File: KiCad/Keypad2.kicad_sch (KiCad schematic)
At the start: 22 parts, among them J1 Keypad, J2 USB-C, U1 ESP32-PICO-MINI-02, U2 SP3485, U3 FT231XQ, U4 LMR16006+FB

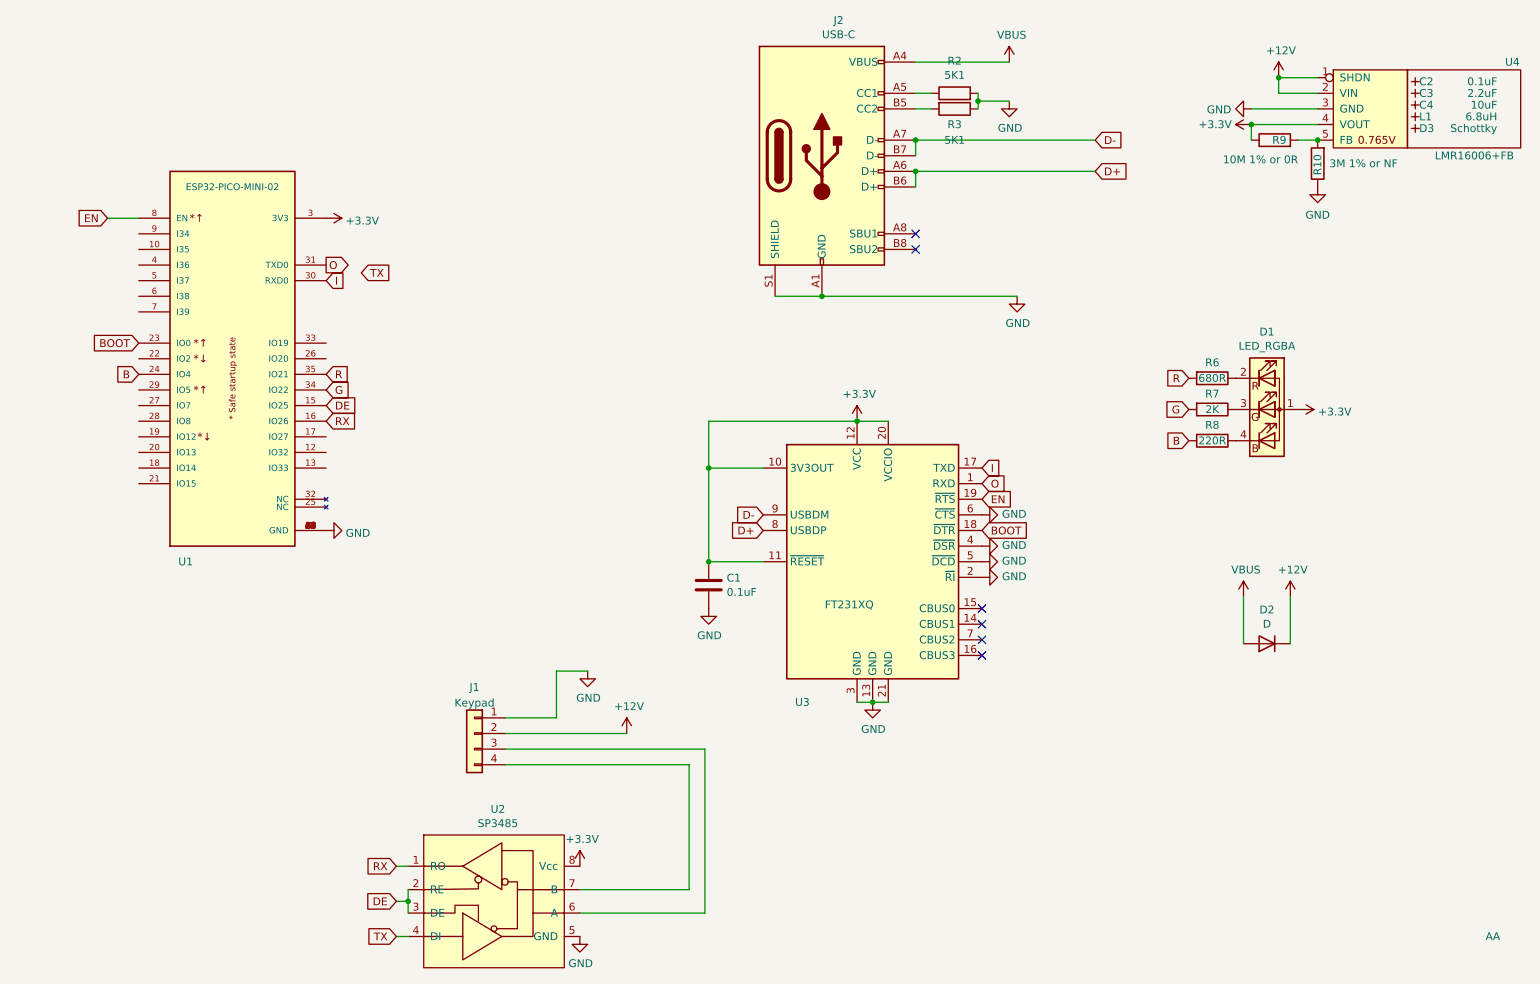
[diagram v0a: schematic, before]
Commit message: Keypad2
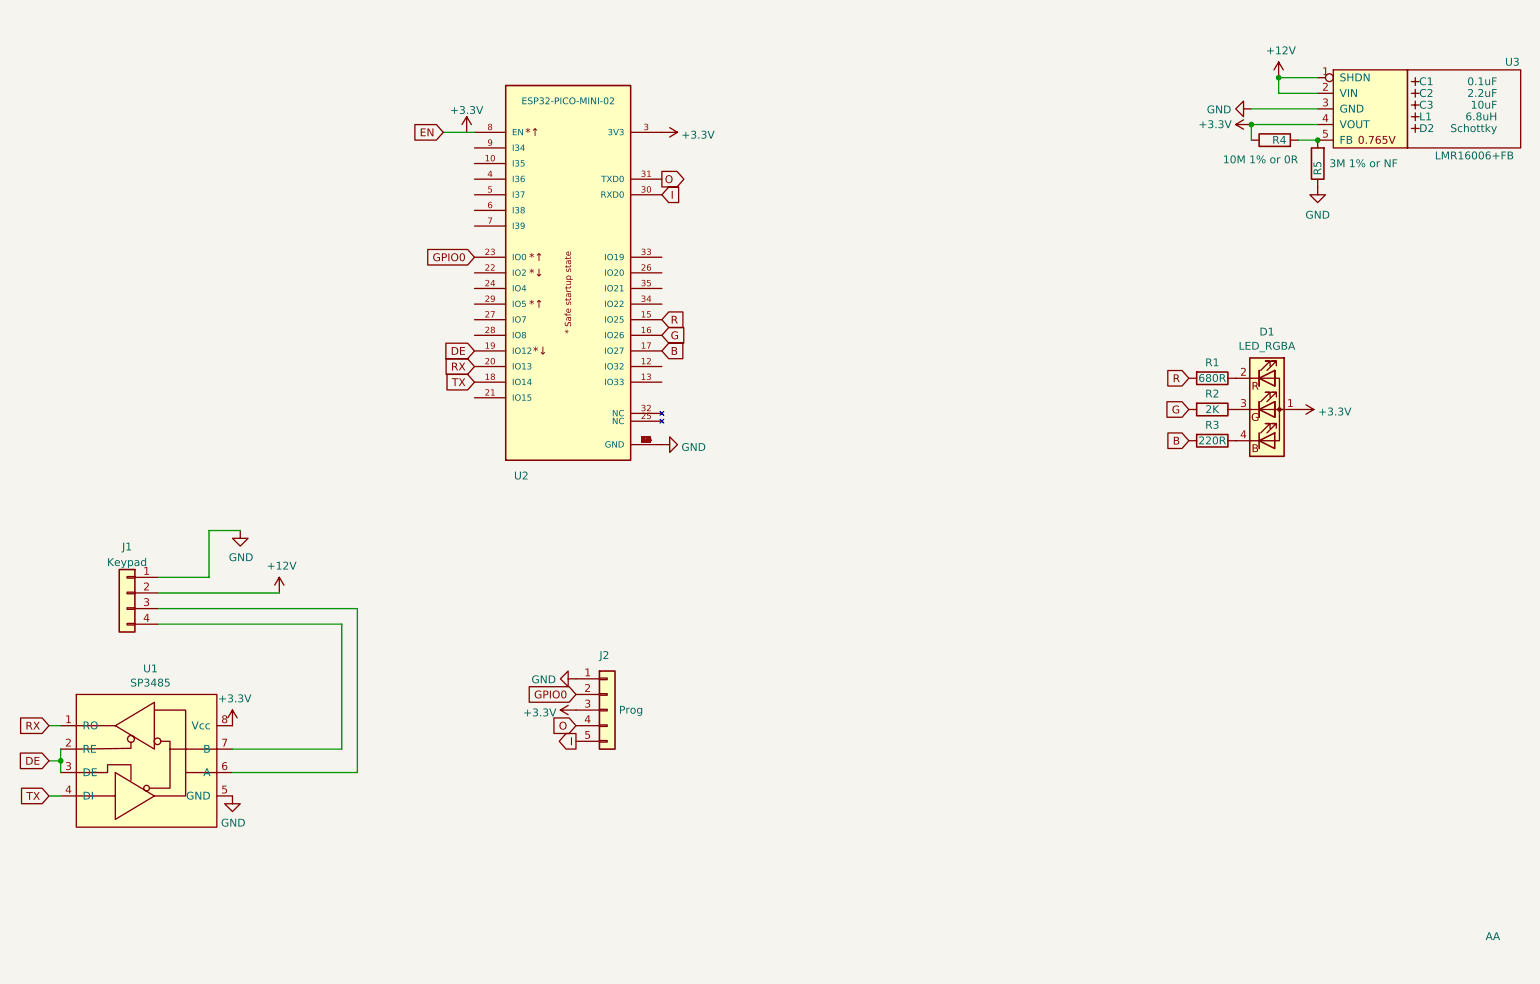
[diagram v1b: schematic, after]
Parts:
- removed C1: 0.1uF, RevK:C_0603, symbol Device:C
- removed D2: D, Diode_SMD:D_1206_3216Metric_Pad1.42x1.75mm_HandSolder, symbol Device:D
- removed J2: USB-C, RevK:USC16-TR-Round, symbol Connector:USB_C_Receptacle_USB2.0
- removed R2, R3: 5K1, RevK:R_0603, symbol Device:R
- removed U3: FT231XQ, RevK:QFN-20-1EP_4x4mm_P0.5mm_EP2.5x2.5mm, symbol Interface_USB:FT231XQ
- added J2: Prog, Connector_PinHeader_2.54mm:PinHeader_1x05_P2.54mm_Vertical, symbol Connector_Generic:Conn_01x05
- renumbered C2 to C1, C3 to C2, C4 to C3, D3 to D2, R6 to R1, R7 to R2, R8 to R3, R9 to R4, R10 to R5, U2 to U1, U1 to U2, U4 to U3
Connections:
- net +3V3: now also J2.3 (Pin_3)
- net B: now also U2.17 (IO27); no longer U2.24 (IO4)
- net DE: now also U2.19 (IO12); no longer U2.15 (IO25)
- net G: now also U2.16 (IO26); no longer U2.34 (IO22)
- net GND: now also J2.1 (Pin_1)
- net I: now also J2.5 (Pin_5)
- net O: now also J2.4 (Pin_4)
- net R: now also U2.15 (IO25); no longer U2.35 (IO21)
- net RX: now also U2.20 (IO13); no longer U2.16 (IO26)
- net TX: now also U2.18 (IO14)
- net BOOT renamed GPIO0
- net GPIO0: now also J2.2 (Pin_2)
- no-connect marks 6 -> 0
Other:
- moved on the sheet: J1, U1, U2
